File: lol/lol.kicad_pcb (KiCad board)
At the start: 2 copper layers, 7.5 x 2 mm, 20 parts, among them J1 USB_B_Micro, J2 5V_BUS, J3 GP_IO, SW1 SW_Push, SW2 SW_Push, SW3 SW_Push, U1 ATmega32U4-MU, Y1 16MHz

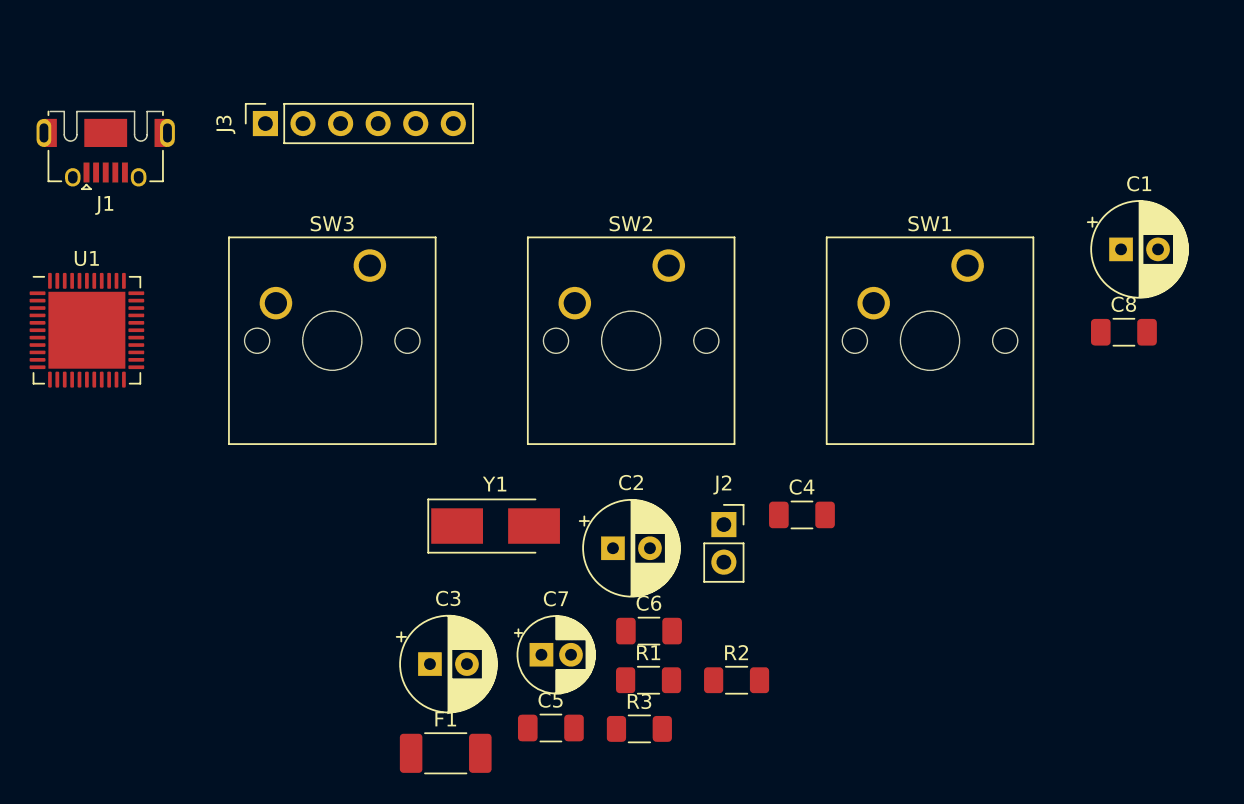
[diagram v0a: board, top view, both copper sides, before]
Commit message: finished pcb... tired....
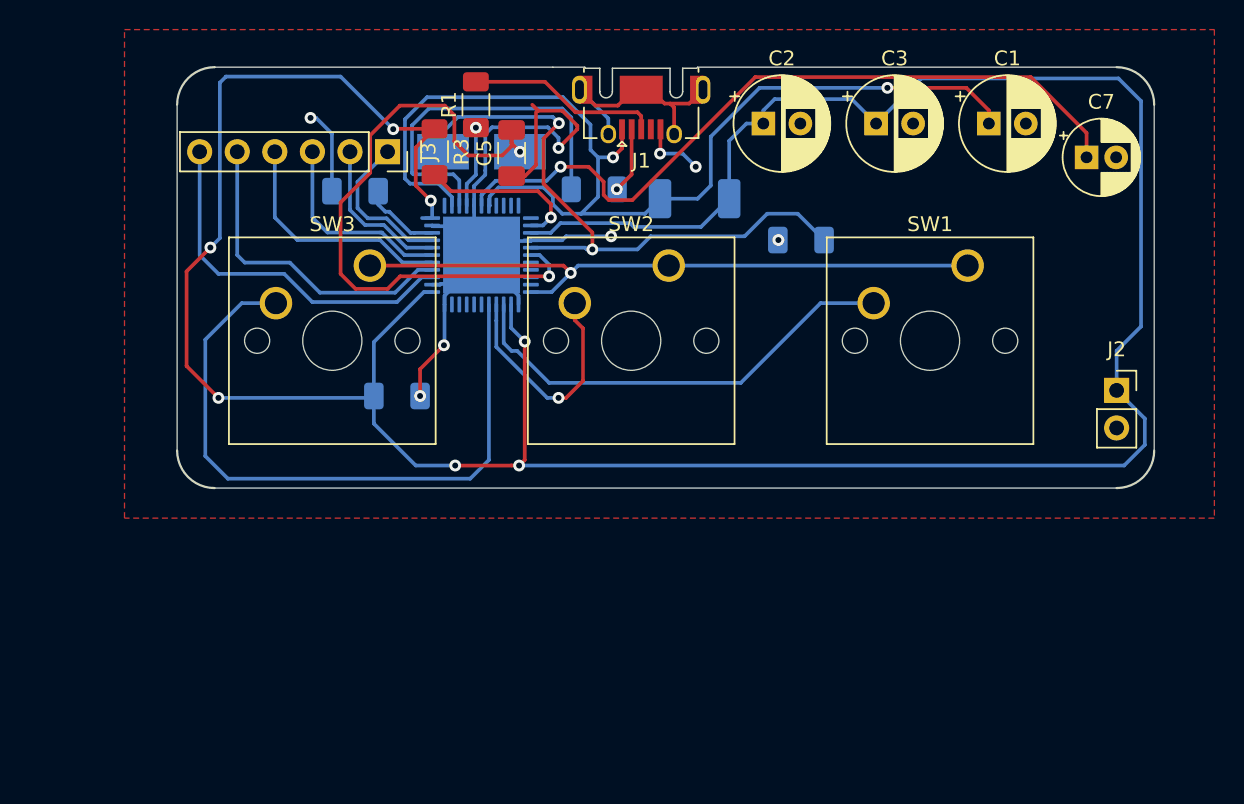
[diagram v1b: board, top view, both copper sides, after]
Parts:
- C4, C6, C8, F1, R2, U1, Y1: moved to B.Cu
- moved C8 52.8 mm to (94.3, 38.9), turned to 180 degrees
- moved C7 49.9 mm to (143.8, 36.6)
- moved C3 47.4 mm to (129.5, 34.3)
- moved R3 41.4 mm to (99.7, 36.2), turned to 270 degrees
- moved F1 41.1 mm to (117.3, 39.4), turned to 180 degrees
- moved R1 40.6 mm to (102.5, 33.0), turned to 90 degrees
- moved C5 39.0 mm to (104.9, 36.3), turned to 90 degrees
- moved J1 36.3 mm to (113.7, 32.0)
- moved R2 34.5 mm to (110.5, 38.7)
- moved C2 30.5 mm to (121.9, 34.3)
- moved C4 28.5 mm to (97.2, 52.7)
- moved C6 28.4 mm to (124.5, 42.2)
- moved J2 28.1 mm to (145.8, 52.3)
- moved U1 27.1 mm to (102.9, 43.2), turned to 270 degrees
- moved Y1 25.3 mm to (102.9, 36.2), turned to 180 degrees
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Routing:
- net VCC: track 0.00 -> 209.0 mm, vias 0 -> 7
- net USB_VBUS: track 0.00 -> 74.8 mm, vias 0 -> 2
- net GND: track 0.00 -> 70.2 mm, vias 0 -> 8
- net Net-(C7-Pad1): track 0.00 -> 50.5 mm, vias 0 -> 1
- net COL3: track 0.00 -> 44.5 mm
- net ROW1: track 0.00 -> 44.0 mm, vias 0 -> 1
- net Net-(C5-Pad2): track 0.00 -> 43.2 mm, vias 0 -> 2
- net Net-(C6-Pad2): track 0.00 -> 41.7 mm, vias 0 -> 2
- net COL1: track 0.00 -> 31.0 mm
- net Net-(J3-Pad6): track 0.00 -> 24.7 mm
- net D-: track 0.00 -> 24.7 mm
- net Net-(J3-Pad5): track 0.00 -> 21.8 mm
- net Net-(J1-Pad6): track 0.00 -> 16.9 mm
- net Net-(J3-Pad4): track 0.00 -> 16.3 mm
- net COL2: track 0.00 -> 16.1 mm, vias 0 -> 1
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- added copper zone on F.Cu, net GND
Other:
- board size 7.5 x 2 mm -> 66 x 28.4 mm
